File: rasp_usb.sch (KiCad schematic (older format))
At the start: 22 parts, among them J1 USB_B_Micro, J2 Conn_02x05_Odd_Even, U1 AMS1117-5.0, U3 CP2104

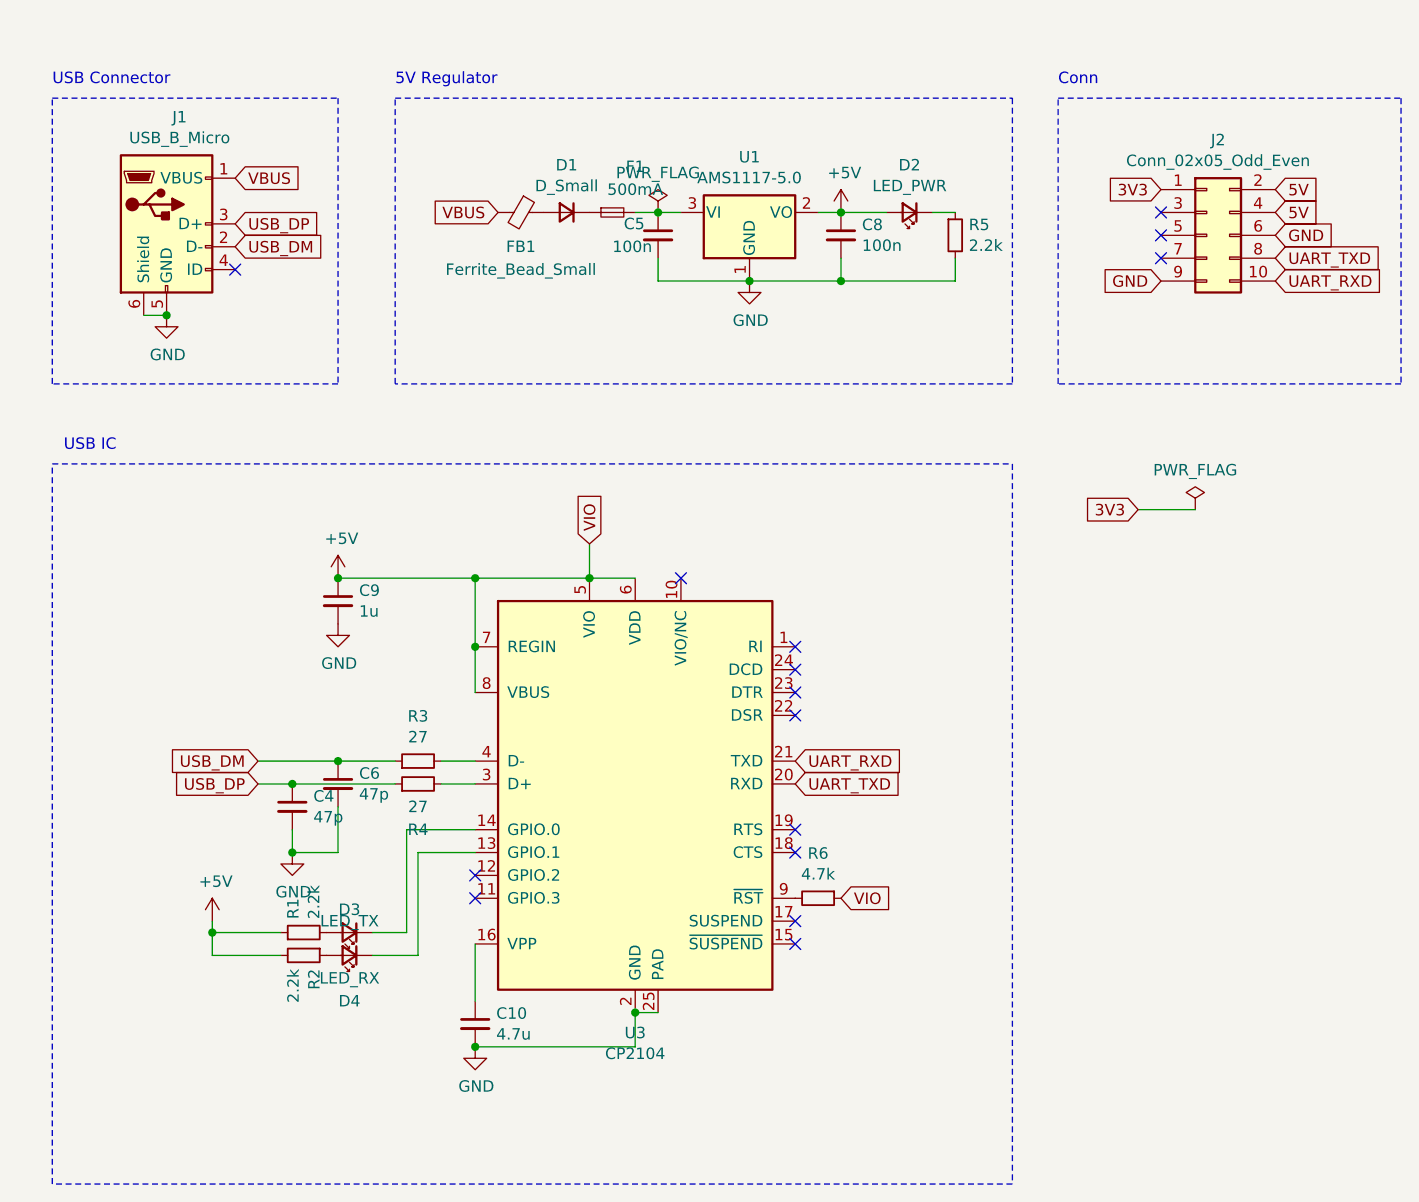
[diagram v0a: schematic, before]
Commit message: Updated schematics as hierarchical structure
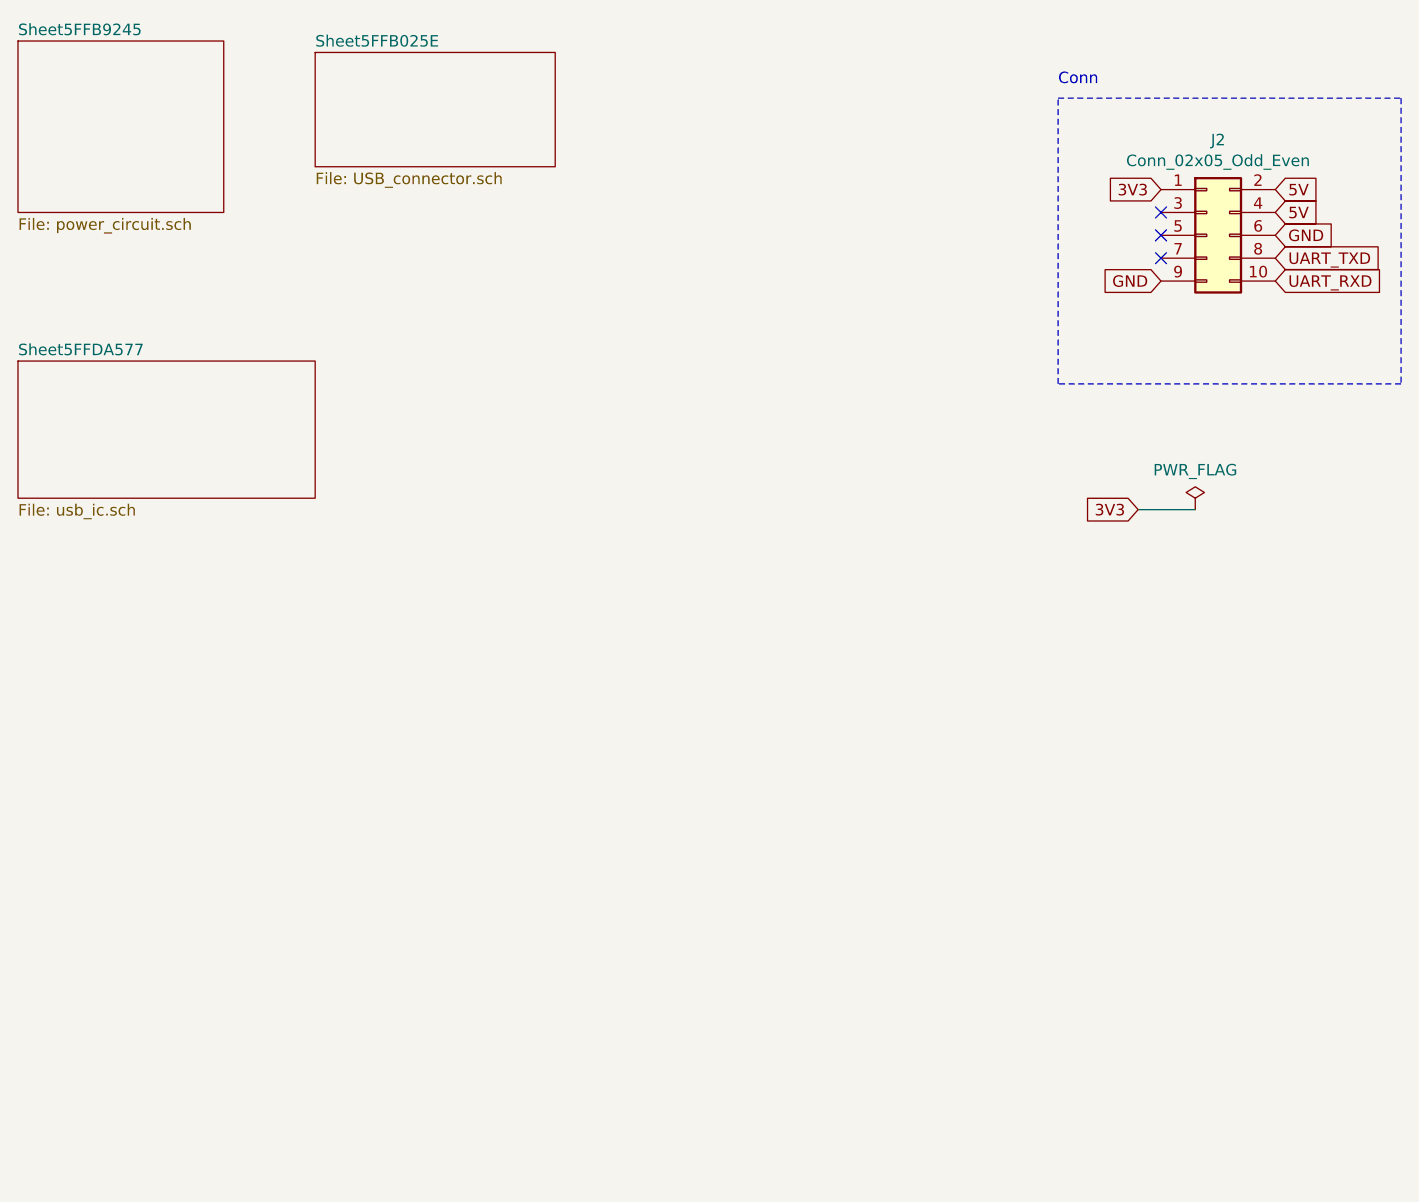
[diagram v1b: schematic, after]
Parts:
- removed C10: 4.7u, Capacitor_SMD:C_0603_1608Metric, symbol Device:C_Small
- removed C4, C6: 47p, Capacitor_SMD:C_0402_1005Metric, symbol Device:C_Small
- removed C5, C8: 100n, Capacitor_SMD:C_0603_1608Metric, symbol Device:C_Small
- removed C9: 1u, Capacitor_SMD:C_0603_1608Metric, symbol Device:C_Small
- removed D1: D_Small, Diode_SMD:D_SOD-123, symbol Device:D_Small
- removed D2: LED_PWR, LED_SMD:LED_0402_1005Metric, symbol Device:LED_Small
- removed D3: LED_TX, LED_SMD:LED_0402_1005Metric, symbol Device:LED_Small
- removed D4: LED_RX, LED_SMD:LED_0402_1005Metric, symbol Device:LED_Small
- removed F1: 500mA, Fuse:Fuse_0603_1608Metric, symbol Device:Fuse_Small
- removed FB1: Ferrite_Bead_Small, Inductor_SMD:L_0603_1608Metric, symbol Device:Ferrite_Bead_Small
- removed J1: USB_B_Micro, Connector_USB:USB_Micro-B_Amphenol_10104110_Horizontal, symbol Connector:USB_B_Micro
- removed R1, R2, R5: 2.2k, Resistor_SMD:R_0402_1005Metric, symbol Device:R_Small
- removed R3, R4: 27, Resistor_SMD:R_0402_1005Metric, symbol Device:R_Small
- removed R6: 4.7k, Resistor_SMD:R_0402_1005Metric, symbol Device:R_Small
- removed U1: AMS1117-5.0, Package_TO_SOT_SMD:SOT-223-3_TabPin2, symbol Regulator_Linear:AMS1117-5.0
- removed U3: CP2104, Package_DFN_QFN:QFN-24-1EP_4x4mm_P0.5mm_EP2.6x2.6mm, symbol Interface_USB:CP2104
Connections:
- no-connect marks 15 -> 3
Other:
- note removed: "5V Regulator"
- note removed: "USB Connector"
- note removed: "USB IC"

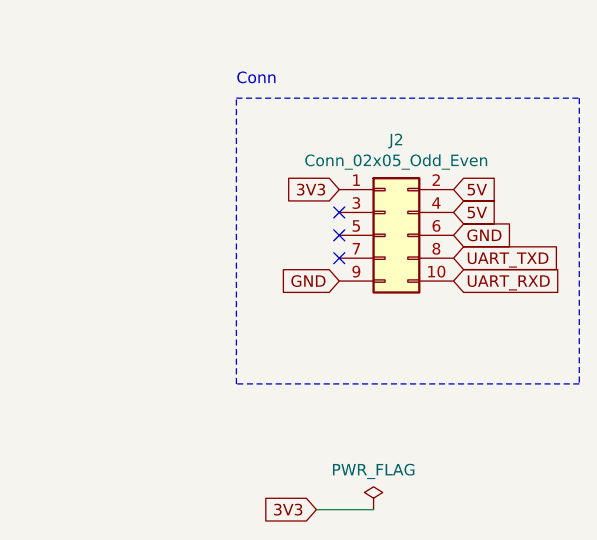
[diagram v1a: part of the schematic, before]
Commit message: annotation number
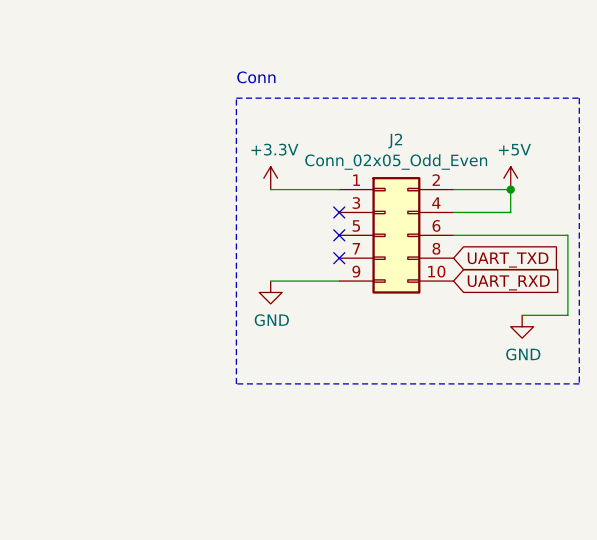
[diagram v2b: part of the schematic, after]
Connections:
- net 3V3 renamed +3V3
- net 5V renamed +5V
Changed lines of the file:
@@
 	1    0    0    -1
 $EndComp
-Text GLabel 6350 1500 2    50   Input ~ 0
-5V
-Text GLabel 6350 1700 2    50   Input ~ 0
-GND
 Text GLabel 6350 1800 2    50   Input ~ 0
 UART_TXD
 Text GLabel 6350 1900 2    50   Input ~ 0
 UART_RXD
-Text GLabel 5850 1900 0    50   Input ~ 0
-GND
-Text GLabel 5850 1500 0    50   Input ~ 0
-3V3
-Text GLabel 6350 1600 2    50   Input ~ 0
-5V
 NoConn ~ 5850 1600
 NoConn ~ 5850 1700
@@
 Text Notes 5400 1050 0    50   ~ 0
 Conn
-Text GLabel 5750 2900 0    50   Input ~ 0
-3V3
-$Comp
-L power:PWR_FLAG #FLG0102
-U 1 1 5FD5B3BE
-P 6000 2900
-F 0 "#FLG0102" H 6000 2975 50  0001 C CNN
-F 1 "PWR_FLAG" H 6000 3073 50  0000 C CNN
-F 2 "" H 6000 2900 50  0001 C CNN
-F 3 "~" H 6000 2900 50  0001 C CNN
-	1    6000 2900
-	1    0    0    -1
-$EndComp
-Wire Wire Line
-	5750 2900 6000 2900
 $Sheet
 S 2150 900  1050 500
@@
 F1 "usb_ic.sch" 50
 $EndSheet
+$Comp
+L power:+5V #PWR0110
+U 1 1 5FFC6082
+P 6600 1500
+F 0 "#PWR0110" H 6600 1350 50  0001 C CNN
+F 1 "+5V" H 6615 1673 50  0000 C CNN
+F 2 "" H 6600 1500 50  0001 C CNN
+F 3 "" H 6600 1500 50  0001 C CNN
+	1    6600 1500
+	1    0    0    -1
+$EndComp
+Wire Wire Line
+	6350 1500 6600 1500
+Wire Wire Line
+	6350 1600 6600 1600
+Wire Wire Line
+	6600 1600 6600 1500
+Connection ~ 6600 1500
+$Comp
+L power:+3.3V #PWR0111
+U 1 1 5FFC6F8E
+P 5550 1500
+F 0 "#PWR0111" H 5550 1350 50  0001 C CNN
+F 1 "+3.3V" H 5565 1673 50  0000 C CNN
+F 2 "" H 5550 1500 50  0001 C CNN
+F 3 "" H 5550 1500 50  0001 C CNN
+	1    5550 1500
+	1    0    0    -1
+$EndComp
+Wire Wire Line
+	5550 1500 5850 1500
+$Comp
+L power:GND #PWR0112
+U 1 1 5FFC7D97
+P 5550 1900
+F 0 "#PWR0112" H 5550 1650 50  0001 C CNN
+F 1 "GND" H 5555 1727 50  0000 C CNN
+F 2 "" H 5550 1900 50  0001 C CNN
+F 3 "" H 5550 1900 50  0001 C CNN
+	1    5550 1900
+	1    0    0    -1
+$EndComp
+Wire Wire Line
+	5850 1900 5550 1900
+$Comp
+L power:GND #PWR0113
+U 1 1 5FFC88A9
+P 6650 2050
+F 0 "#PWR0113" H 6650 1800 50  0001 C CNN
+F 1 "GND" H 6655 1877 50  0000 C CNN
+F 2 "" H 6650 2050 50  0001 C CNN
+F 3 "" H 6650 2050 50  0001 C CNN
+	1    6650 2050
+	1    0    0    -1
+$EndComp
+Wire Wire Line
+	6350 1700 6850 1700
+Wire Wire Line
+	6850 1700 6850 2050
+Wire Wire Line
+	6850 2050 6650 2050
 $EndSCHEMATC

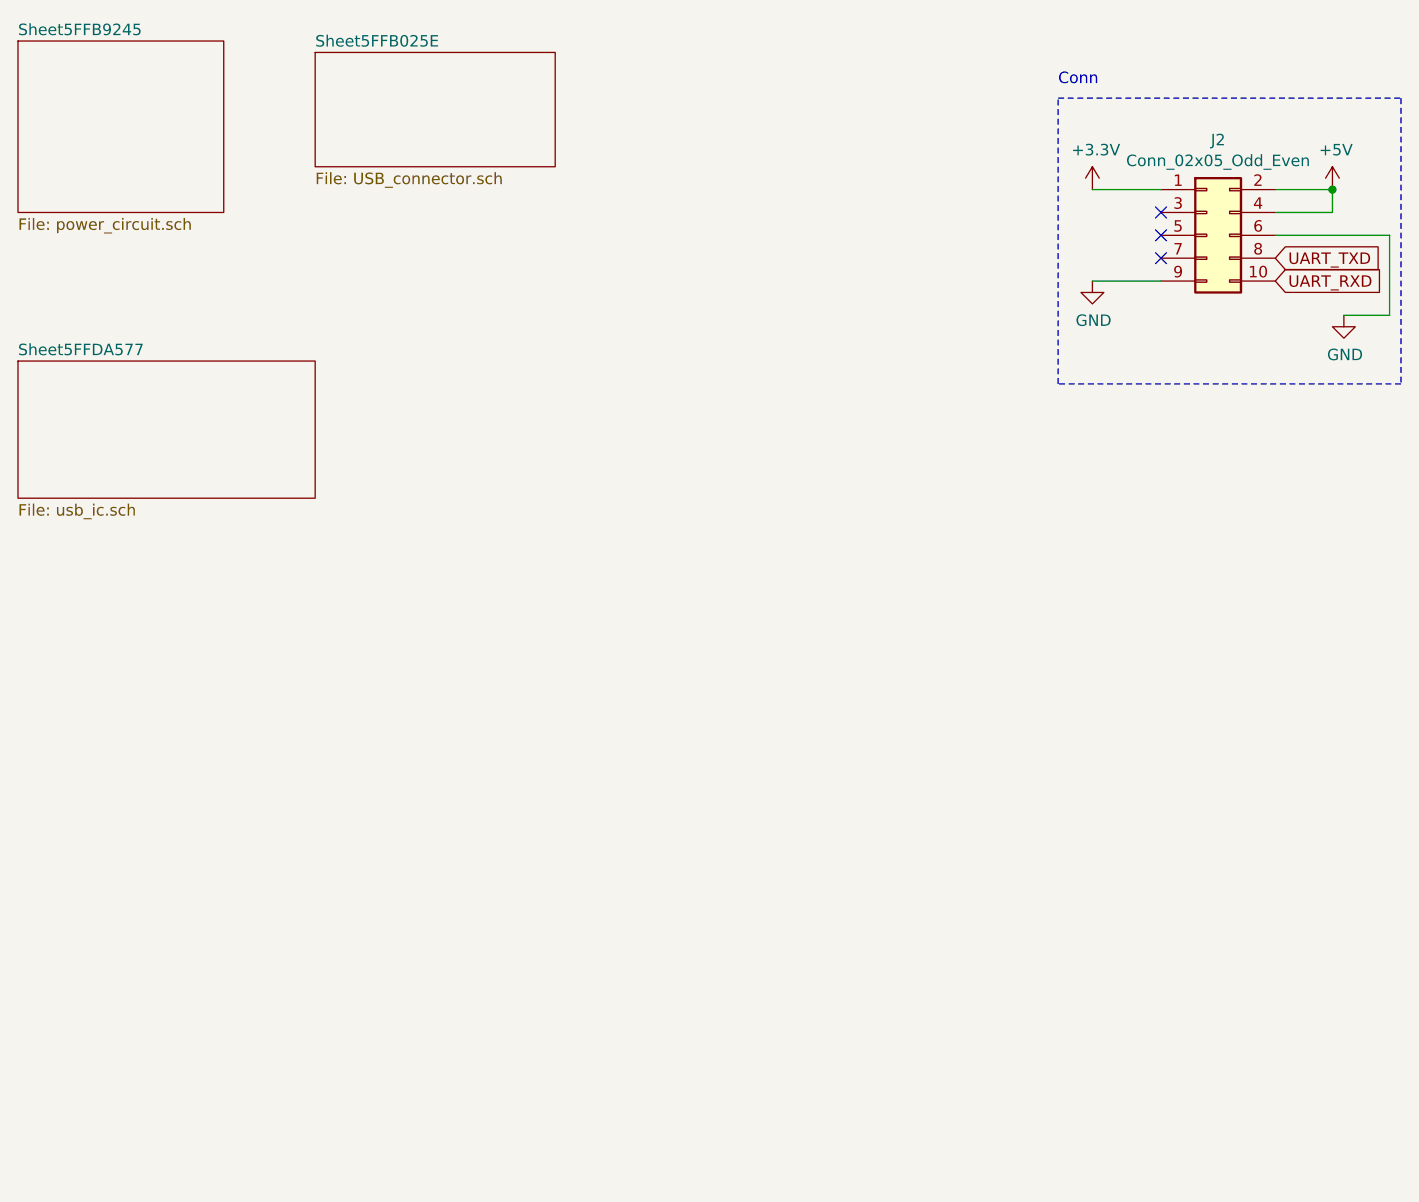
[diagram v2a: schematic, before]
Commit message: Ready to order
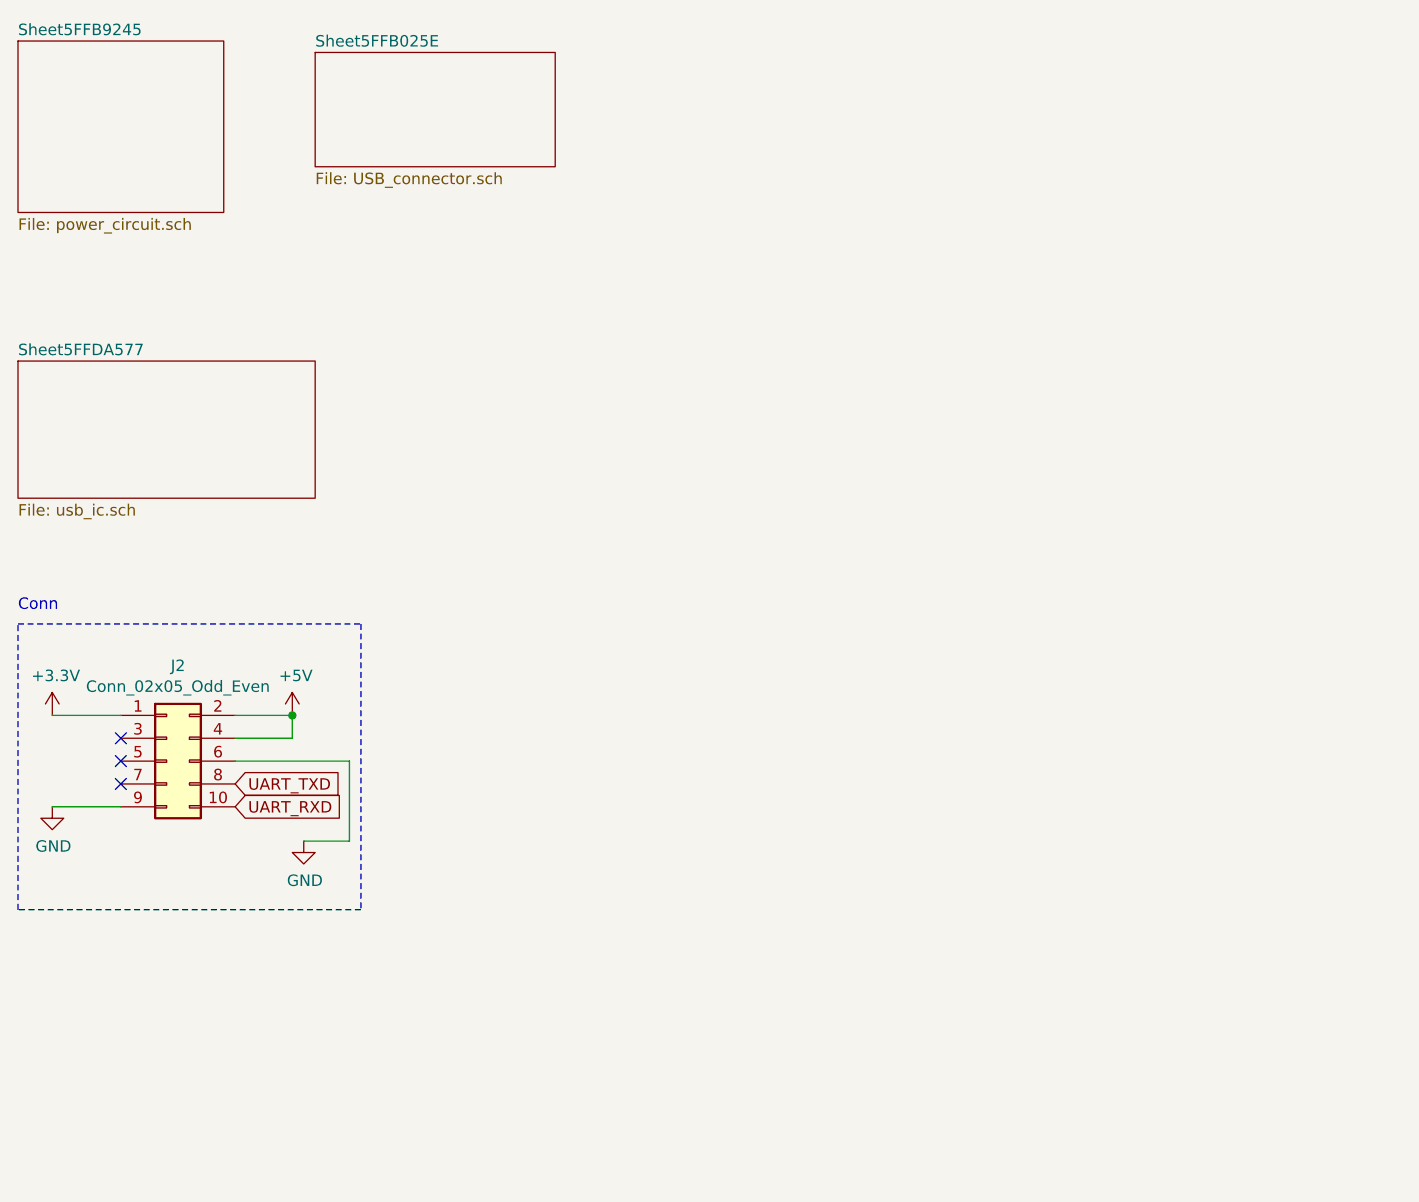
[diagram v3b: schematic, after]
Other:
- moved on the sheet: J2
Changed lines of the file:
@@
 L Connector_Generic:Conn_02x05_Odd_Even J2
 U 1 1 5FBEC2E7
-P 6050 1700
-F 0 "J2" H 6100 2117 50  0000 C CNN
-F 1 "Conn_02x05_Odd_Even" H 6100 2026 50  0000 C CNN
-F 2 "Connector_PinSocket_2.54mm:PinSocket_2x05_P2.54mm_Vertical" H 6050 1700 50  0001 C CNN
-F 3 "~" H 6050 1700 50  0001 C CNN
-	1    6050 1700
+P 1500 4000
+F 0 "J2" H 1550 4417 50  0000 C CNN
+F 1 "Conn_02x05_Odd_Even" H 1550 4326 50  0000 C CNN
+F 2 "Connector_PinSocket_2.54mm:PinSocket_2x05_P2.54mm_Vertical" H 1500 4000 50  0001 C CNN
+F 3 "~" H 1500 4000 50  0001 C CNN
+	1    1500 4000
 	1    0    0    -1
 $EndComp
-Text GLabel 6350 1800 2    50   Input ~ 0
+Text GLabel 1800 4100 2    50   Input ~ 0
 UART_TXD
-Text GLabel 6350 1900 2    50   Input ~ 0
+Text GLabel 1800 4200 2    50   Input ~ 0
 UART_RXD
-NoConn ~ 5850 1600
-NoConn ~ 5850 1700
-NoConn ~ 5850 1800
+NoConn ~ 1300 3900
+NoConn ~ 1300 4000
+NoConn ~ 1300 4100
 Wire Notes Line
-	5400 1100 6900 1100
+	850  3400 2350 3400
 Wire Notes Line
-	6900 1100 6900 2350
+	2350 3400 2350 4650
 Wire Notes Line
-	6900 2350 5400 2350
+	2350 4650 850  4650
 Wire Notes Line
-	5400 2350 5400 1100
-Text Notes 5400 1050 0    50   ~ 0
+	850  4650 850  3400
+Text Notes 850  3350 0    50   ~ 0
 Conn
 $Sheet
@@
 L power:+5V #PWR0110
 U 1 1 5FFC6082
-P 6600 1500
-F 0 "#PWR0110" H 6600 1350 50  0001 C CNN
-F 1 "+5V" H 6615 1673 50  0000 C CNN
-F 2 "" H 6600 1500 50  0001 C CNN
-F 3 "" H 6600 1500 50  0001 C CNN
-	1    6600 1500
+P 2050 3800
+F 0 "#PWR0110" H 2050 3650 50  0001 C CNN
+F 1 "+5V" H 2065 3973 50  0000 C CNN
+F 2 "" H 2050 3800 50  0001 C CNN
+F 3 "" H 2050 3800 50  0001 C CNN
+	1    2050 3800
 	1    0    0    -1
 $EndComp
 Wire Wire Line
-	6350 1500 6600 1500
+	1800 3800 2050 3800
 Wire Wire Line
-	6350 1600 6600 1600
+	1800 3900 2050 3900
 Wire Wire Line
-	6600 1600 6600 1500
-Connection ~ 6600 1500
+	2050 3900 2050 3800
+Connection ~ 2050 3800
 $Comp
 L power:+3.3V #PWR0111
 U 1 1 5FFC6F8E
-P 5550 1500
-F 0 "#PWR0111" H 5550 1350 50  0001 C CNN
-F 1 "+3.3V" H 5565 1673 50  0000 C CNN
-F 2 "" H 5550 1500 50  0001 C CNN
-F 3 "" H 5550 1500 50  0001 C CNN
-	1    5550 1500
+P 1000 3800
+F 0 "#PWR0111" H 1000 3650 50  0001 C CNN
+F 1 "+3.3V" H 1015 3973 50  0000 C CNN
+F 2 "" H 1000 3800 50  0001 C CNN
+F 3 "" H 1000 3800 50  0001 C CNN
+	1    1000 3800
 	1    0    0    -1
 $EndComp
 Wire Wire Line
-	5550 1500 5850 1500
+	1000 3800 1300 3800
 $Comp
 L power:GND #PWR0112
 U 1 1 5FFC7D97
-P 5550 1900
-F 0 "#PWR0112" H 5550 1650 50  0001 C CNN
-F 1 "GND" H 5555 1727 50  0000 C CNN
-F 2 "" H 5550 1900 50  0001 C CNN
-F 3 "" H 5550 1900 50  0001 C CNN
-	1    5550 1900
+P 1000 4200
+F 0 "#PWR0112" H 1000 3950 50  0001 C CNN
+F 1 "GND" H 1005 4027 50  0000 C CNN
+F 2 "" H 1000 4200 50  0001 C CNN
+F 3 "" H 1000 4200 50  0001 C CNN
+	1    1000 4200
 	1    0    0    -1
 $EndComp
 Wire Wire Line
-	5850 1900 5550 1900
+	1300 4200 1000 4200
 $Comp
 L power:GND #PWR0113
 U 1 1 5FFC88A9
-P 6650 2050
-F 0 "#PWR0113" H 6650 1800 50  0001 C CNN
-F 1 "GND" H 6655 1877 50  0000 C CNN
-F 2 "" H 6650 2050 50  0001 C CNN
-F 3 "" H 6650 2050 50  0001 C CNN
-	1    6650 2050
+P 2100 4350
+F 0 "#PWR0113" H 2100 4100 50  0001 C CNN
+F 1 "GND" H 2105 4177 50  0000 C CNN
+F 2 "" H 2100 4350 50  0001 C CNN
+F 3 "" H 2100 4350 50  0001 C CNN
+	1    2100 4350
 	1    0    0    -1
 $EndComp
 Wire Wire Line
-	6350 1700 6850 1700
+	1800 4000 2300 4000
 Wire Wire Line
-	6850 1700 6850 2050
+	2300 4000 2300 4350
 Wire Wire Line
-	6850 2050 6650 2050
+	2300 4350 2100 4350
 $EndSCHEMATC
